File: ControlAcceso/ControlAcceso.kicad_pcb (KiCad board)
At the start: 2 copper layers, 53.3 x 61 mm, 14 parts, among them U1 LM7805_TO220

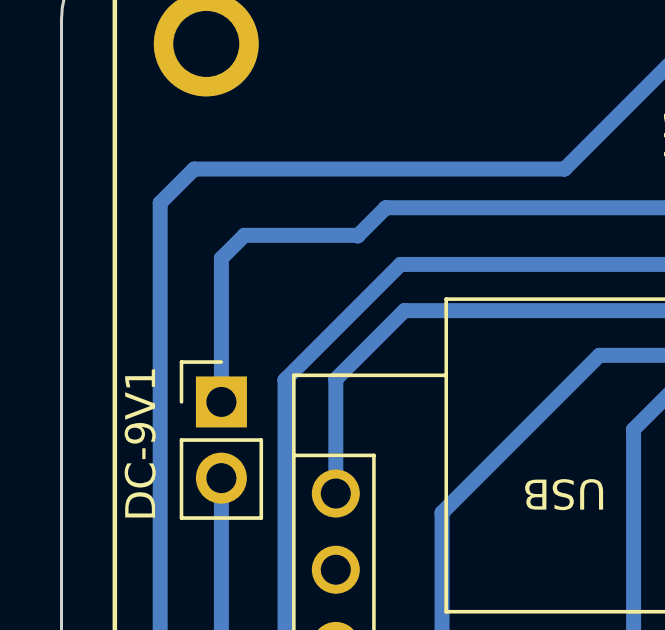
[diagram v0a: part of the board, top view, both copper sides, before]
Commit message: Modificaciones Varias
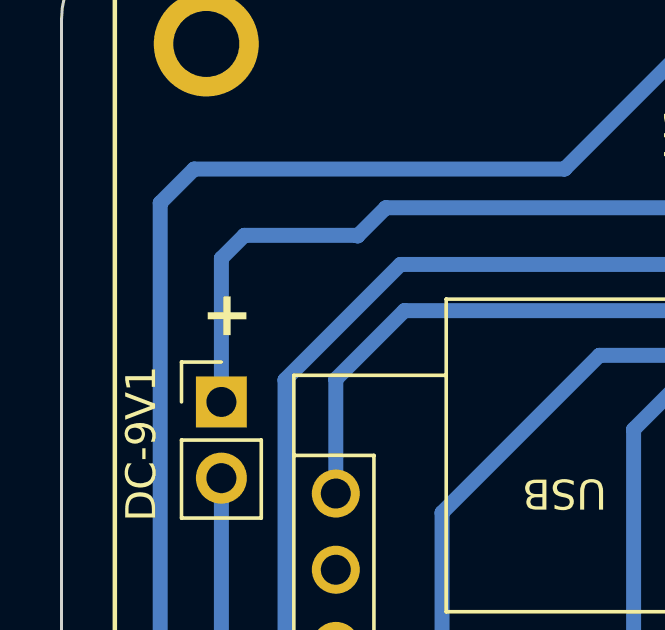
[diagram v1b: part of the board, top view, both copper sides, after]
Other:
- board text added: "+"
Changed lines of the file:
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@@
     (pad_to_mask_clearance 0)
     (pcbplotparams
-      (layerselection 0x00010fc_ffffffff)
+      (layerselection 0x0001000_ffffffff)
       (plot_on_all_layers_selection 0x0000000_00000000)
       (disableapertmacros false)
@@
       (net 25 "Net-(D2-A)") (pinfunction "A") (pintype "passive"))
     (model "${KICAD6_3DMODEL_DIR}/LED_THT.3dshapes/LED_D5.0mm.wrl"
-      (offset (xyz 0 0 0))
+      (offset (xyz 0 0 -3))
       (scale (xyz 1 1 1))
       (rotate (xyz 0 0 0))
@@
       (net 24 "Net-(D1-A)") (pinfunction "A") (pintype "passive"))
     (model "${KICAD6_3DMODEL_DIR}/LED_THT.3dshapes/LED_D5.0mm.wrl"
-      (offset (xyz 0 0 0))
+      (offset (xyz 0 0 -3))
       (scale (xyz 1 1 1))
       (rotate (xyz 0 0 0))
@@
     (pad "30" thru_hole oval (at 15.24 0 180) (size 1.6 1.6) (drill 1) (layers "*.Cu" "*.Mask")
       (net 23 "VIN") (pinfunction "VIN") (pintype "power_in"))
-    (model "C:/Users/hjest/Downloads/arduino-nano-33-iot-1.snapshot.3/Arduino Nano 33 IoT.stp"
-      (offset (xyz 7.5 -17.5 0.5))
+    (model "C:/Users/RED-TECNOPARQUE/Downloads/arduino-nano-33-iot-1.snapshot.3/Arduino Nano 33 IoT.stp"
+      (opacity 0.9900)      (offset (xyz 7.5 -17.5 1.5))
       (scale (xyz 1 1 1))
-      (rotate (xyz -90 0 0))
+      (rotate (xyz 90 -180 -180))
     )
   )
@@
     (pad "VCC1" thru_hole circle (at 13.97 7.62 90) (size 1.108 1.108) (drill 0.6) (layers "*.Cu" "*.Mask")
       (net 28 "unconnected-(RDM1-PadVCC1)") (pinfunction "VCC1") (pintype "bidirectional") (solder_mask_margin 0.102))
-    (model "C:/Users/hjest/Downloads/RDM6300/RDM6300.step"
-      (offset (xyz 0 0 5))
+    (model "C:/Users/RED-TECNOPARQUE/Downloads/rdm6300-4.snapshot.1/RDM6300.step"
+      (offset (xyz 0 0 4.5))
       (scale (xyz 1 1 1))
       (rotate (xyz 0 0 90))
@@
     (pad "3" thru_hole oval (at 5.08 0 90) (size 1.905 2) (drill 1.1) (layers "*.Cu" "*.Mask")
       (net 23 "VIN") (pinfunction "VO") (pintype "power_out"))
-    (model "C:/Users/hjest/Downloads/7805-3.snapshot.1/7805BC/7805BC.stp"
-      (offset (xyz 2.5 9 0.5))
+    (model "C:/Users/RED-TECNOPARQUE/Downloads/7805-3.snapshot.1/7805BC/7805BC.stp"
+      (offset (xyz 2.5 9 0))
       (scale (xyz 1 1 1))
       (rotate (xyz 0 0 0))
@@
     (effects (font (size 1 1) (thickness 0.2) bold) (justify left bottom))
   )
+  (gr_text "+\n" (at 199.42 49.26) (layer "F.SilkS")
+    (effects (font (size 1.5 1.5) (thickness 0.3) bold) (justify left bottom mirror))
+  )
   (gr_text "nodo Pitalito" (at 199.119622 65.980851 90) (layer "F.SilkS")
     (effects (font (size 0.677407 0.609666) (thickness 0.084675)) (justify left bottom))
@@
     (effects (font (size 0.7 0.7) (thickness 0.15)) (justify left bottom))
   )
+  (dimension (type aligned) (layer "User.1")
+    (pts (xy 235.36 35.6) (xy 235.4 96.58))
+    (height -24.775437)
+    (gr_text "60,9800 mm" (at 261.955432 66.072567 270.0375833) (layer "User.1")
+      (effects (font (size 1.5 1.5) (thickness 0.3)))
+    )
+    (format (prefix "") (suffix "") (units 3) (units_format 1) (precision 4))
+    (style (thickness 0.2) (arrow_length 1.27) (text_position_mode 0) (extension_height 0.58642) (extension_offset 0.5) keep_text_aligned)
+  )
+  (dimension (type aligned) (layer "User.1")
+    (pts (xy 246.38 38.56) (xy 193.04 38.56))
+    (height 8.87)
+    (gr_text "53,3400 mm" (at 219.71 27.89) (layer "User.1")
+      (effects (font (size 1.5 1.5) (thickness 0.3)))
+    )
+    (format (prefix "") (suffix "") (units 3) (units_format 1) (precision 4))
+    (style (thickness 0.2) (arrow_length 1.27) (text_position_mode 0) (extension_height 0.58642) (extension_offset 0.5) keep_text_aligned)
+  )
   (segment (start 223.874 36.576) (end 233.934 36.576) (width 0.5) (layer "B.Cu") (net 4))
